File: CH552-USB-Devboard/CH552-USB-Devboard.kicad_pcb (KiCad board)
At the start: 2 copper layers, 22 x 48.1 mm, 42 parts, among them J1 Conn_01x11_Male, J2 Conn_01x11_Male, J3 USB_C_Receptacle, J4 USB_C_Receptacle, SW1 SW_Push, SW2 SW_Push, U1 CH552T, U2 CH552G

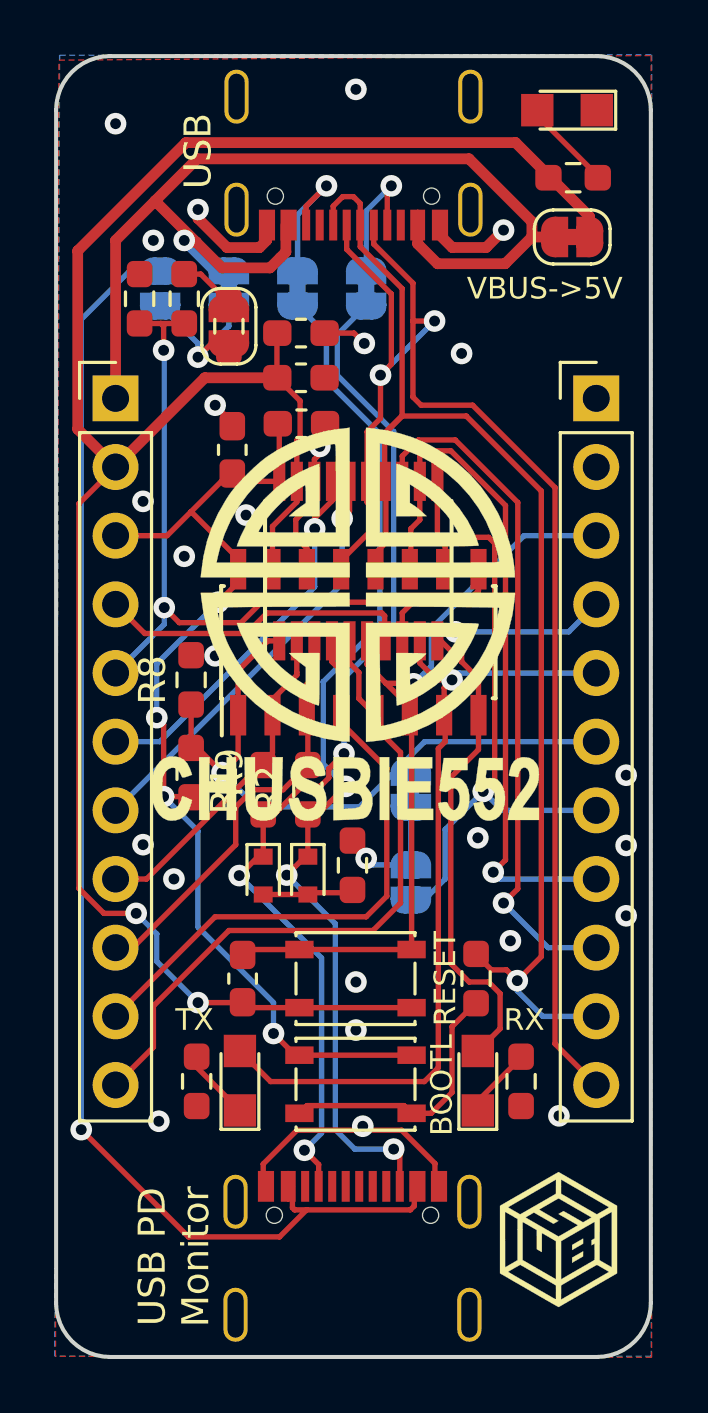
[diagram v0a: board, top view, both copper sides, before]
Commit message: update PCB
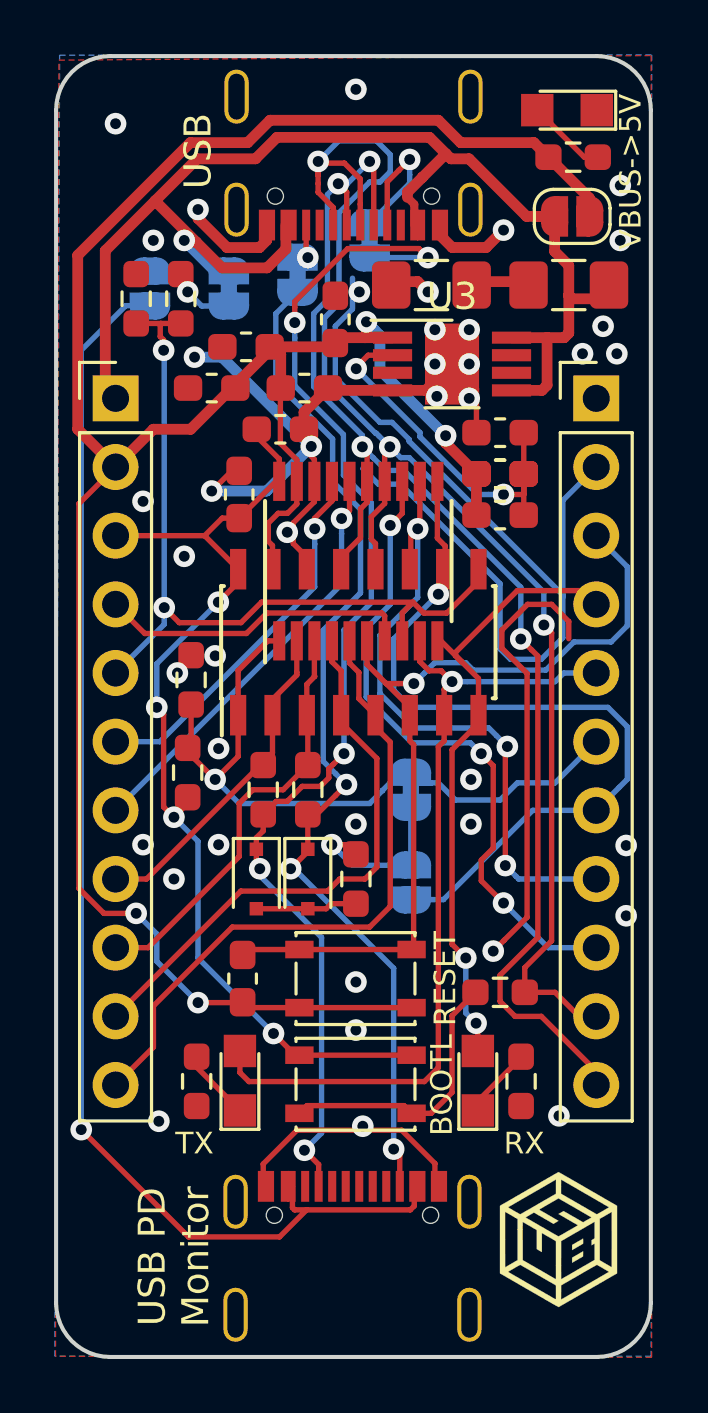
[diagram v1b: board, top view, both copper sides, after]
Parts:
- removed the G*** at (84.7, 84.1)
- removed JP4: Jumper, Jumper:SolderJumper-2_P1.3mm_Open_RoundedPad1.0x1.5mm
- added C10: 10uF, Capacitor_SMD:C_0603_1608Metric_Pad1.05x0.95mm_HandSolder, F.Cu at (83.2, 73.3)
- added C5: 4u7, 50V, Capacitor_SMD:C_1206_3216Metric_Pad1.42x1.75mm_HandSolder, F.Cu at (93.0, 69.5)
- added C6: 4u7, 50V, Capacitor_SMD:C_1206_3216Metric_Pad1.42x1.75mm_HandSolder, F.Cu at (87.9, 69.5)
- added C8: 10nF, Capacitor_SMD:C_0603_1608Metric_Pad1.05x0.95mm_HandSolder, F.Cu at (90.4, 78.0)
- added C9: 100nF, Capacitor_SMD:C_0603_1608Metric_Pad1.05x0.95mm_HandSolder, F.Cu at (84.3, 70.7)
- added R13: 22k, Resistor_SMD:R_0603_1608Metric_Pad1.05x0.95mm_HandSolder, F.Cu at (90.4, 74.9)
- added R14: DNP / 68k, Resistor_SMD:R_0603_1608Metric_Pad1.05x0.95mm_HandSolder, F.Cu at (90.4, 76.5)
- added U3: TPS7A4101DGNT, CH552-USB-Devboard:HVSSOP-8_3.0x3.0mm_P0.65mm, F.Cu at (88.6, 72.4)
- D1, D2: value LED -> LED, yellow
- D3: value LED -> LED, green?
- D4, D5: footprint Diode_SMD:D_SOD-523 -> Diode_SMD:D_SOD-323F
- JP1: footprint Jumper:SolderJumper-2_P1.3mm_Bridged_RoundedPad1.0x1.5mm -> Jumper:SolderJumper-2_P1.3mm_Open_RoundedPad1.0x1.5mm
- R11: value 22k -> 62k; footprint Resistor_SMD:R_0603_1608Metric_Pad0.98x0.95mm_HandSolder -> Resistor_SMD:R_0603_1608Metric_Pad1.05x0.95mm_HandSolder
- R12: value 22k -> 10k
- R3, R4, R5: value 1k -> 10k
- moved R11 11.4 mm to (90.4, 76.5), turned to 180 degrees
- moved C1 3.32 mm to (79.8, 73.3), turned to 180 degrees
- moved C4 2.09 mm to (81.0, 71.8), turned to 180 degrees
- moved JP5 1.78 mm to (85.6, 67.8)
- moved C7 1.67 mm to (80.8, 77.2)
- moved R6 1.02 mm to (90.4, 95.6), turned to 180 degrees
- moved C2 0.81 mm to (82.3, 74.8)
- moved JP1 0.76 mm to (93.1, 66.9)
- moved R5 0.76 mm to (93.1, 64.7)
- moved R7 0.52 mm to (85.1, 91.4)
- moved JP6 0.51 mm to (82.9, 69.1)
- moved JP8 0.38 mm to (77.5, 69.6), turned to 90 degrees
- moved D4 0.28 mm to (81.4, 91.4)
- moved D5 0.13 mm to (83.3, 91.4)
- moved R10 0.13 mm to (77.0, 70.0)
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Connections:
- JP7 pad 2: Net-(JP4-Pad1) -> Net-(JP7-Pad2)
- JP8 pad 2: Net-(JP4-Pad1) -> Net-(JP7-Pad2)
- R11 pad 1: Net-(JP4-Pad2) -> Net-(C8-Pad2)
- R11 pad 2: Net-(JP4-Pad1) -> VCC
- R12 pad 2: Net-(JP4-Pad2) -> Net-(JP7-Pad2)
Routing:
- net GND: track 25.4 -> 96.5 mm, vias 24 -> 41
- net VCC: track 79.3 -> 93.7 mm, vias 2 -> 4
- net Net-(C8-Pad2): track 0.00 -> 13.6 mm, vias 0 -> 2
- net VBUS: track 40.9 -> 50.1 mm
- net /CC1: track 38.8 -> 45.8 mm, vias 3 -> 5
- net Net-(JP4-Pad1): track 6.20 -> 0.00 mm, vias 1 -> 0
- net /P3.6: track 47.9 -> 53.8 mm, vias 1 -> 3
- net /P3.3: track 24.8 -> 29.6 mm
- net Net-(JP7-Pad2): track 0.00 -> 4.17 mm, vias 0 -> 1
- net /P3.7: track 54.4 -> 50.7 mm, vias 2 -> 4
- net Net-(J3-PadB5): track 5.36 -> 1.79 mm
- net /RESET: track 29.2 -> 32.3 mm
- net Net-(JP4-Pad2): track 2.34 -> 0.00 mm
- net /P3.4: track 26.1 -> 23.9 mm, vias 1 -> 3
- net Net-(C5-Pad2): track 0.00 -> 2.11 mm
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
